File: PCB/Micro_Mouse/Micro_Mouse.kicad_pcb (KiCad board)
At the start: 2 copper layers, 88.9 x 91.4 mm, 9 parts, among them J1 Motor Battery Pack, J3 MOT_1/ENC_1, J4 MOT2/ENC_2, J5 TOF, J6 IR_1, J7 IR_2, J8 IMU, U1 TB6612FNG

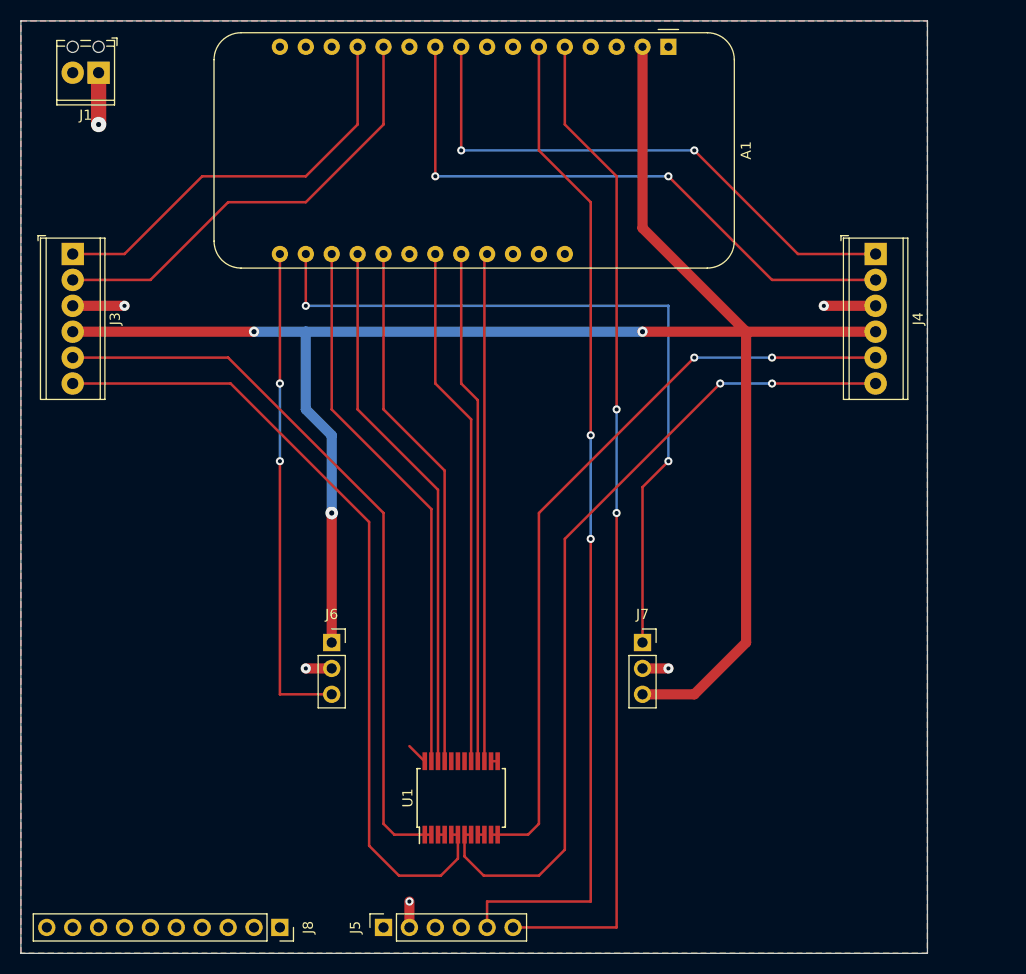
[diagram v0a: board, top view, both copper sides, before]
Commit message: Add files via upload
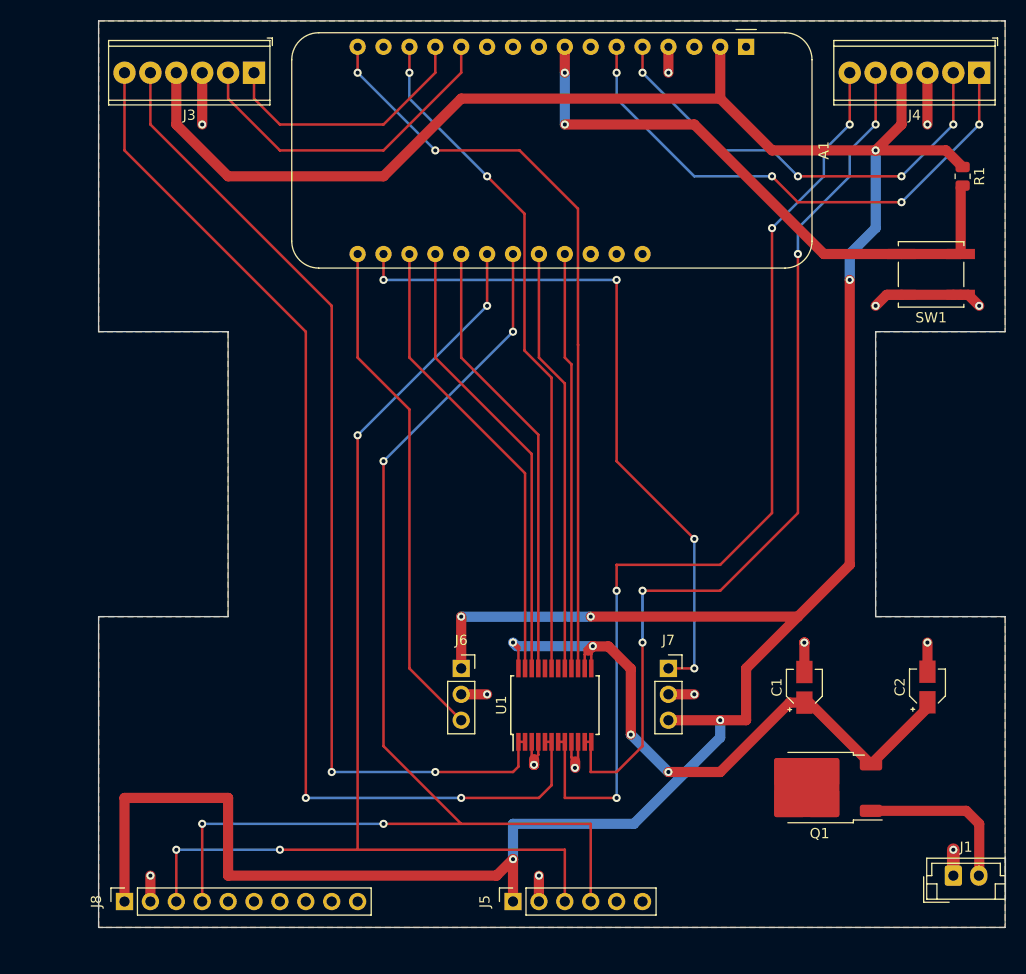
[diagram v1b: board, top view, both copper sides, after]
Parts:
- added C1: 0.1uF, Capacitor_SMD:CP_Elec_3x5.3, F.Cu at (178.4, 116.2)
- added C2: 10uF, Capacitor_SMD:CP_Elec_3x5.3, F.Cu at (190.5, 116.1)
- added Q1: PMOS, Package_TO_SOT_SMD:TO-252-2, F.Cu at (179.9, 126.0)
- added R1: 10K, Resistor_SMD:R_0805_2012Metric, F.Cu at (194.0, 66.0)
- added SW1: Start, Button_Switch_SMD:SW_Push_1P1T_NO_CK_KSC6xxJ, F.Cu at (190.9, 75.7)
- J1: footprint TerminalBlock_Phoenix:TerminalBlock_Phoenix_MPT-0,5-2-2.54_1x02_P2.54mm_Horizontal -> Connector_JST:JST_EH_B2B-EH-A_1x02_P2.50mm_Vertical
- moved J1 115.0 mm to (193.0, 134.6), turned to 0 degrees
- moved J3 25.1 mm to (124.5, 55.9), turned to 180 degrees
- moved J4 20.5 mm to (195.6, 55.9), turned to 180 degrees
- moved J8 15.5 mm to (111.8, 137.2), turned to 90 degrees
- moved J5 13.0 mm to (149.9, 137.2)
- moved J6 13.0 mm to (144.8, 114.3)
- moved U1 12.9 mm to (154.0, 117.9)
- moved A1 7.62 mm to (172.7, 53.3)
- moved J7 3.59 mm to (165.1, 114.3)
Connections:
- net Net-(A1-SCL/IO22) renamed IR_2
- net Net-(A1-SDA/IO23) renamed IR_1
- A1 pad 10: E2_PHA -> unconnected-(A1-IO4/A5-Pad10)
- A1 pad 14: unconnected-(A1-RX/IO16-Pad14) -> STBY
- A1 pad 16: unconnected-(A1-IO21-Pad16) -> PWMB
- A1 pad 22: unconnected-(A1-A9/IO33-Pad22) -> I2C SCL
- A1 pad 23: BIN1 -> I2C SDA
- A1 pad 24: BIN2 -> BIN1
- A1 pad 25: PWMB -> BIN2
- A1 pad 5: Net-(A1-DAC2/A0) -> E2_PHA
- A1 pad 6: Net-(A1-DAC1/A1) -> E2_PHB
- A1 pad 8: unconnected-(A1-I39/A3-Pad8) -> BTN
- A1 pad 9: E2_PHB -> unconnected-(A1-IO36/A4-Pad9)
- J5 pad 3: unconnected-(J5-Pin_3-Pad3) -> I2C SCL
- J5 pad 4: unconnected-(J5-Pin_4-Pad4) -> I2C SDA
- J5 pad 5: Net-(A1-DAC1/A1) -> unconnected-(J5-Pin_5-Pad5)
- J5 pad 6: Net-(A1-DAC2/A0) -> unconnected-(J5-Pin_6-Pad6)
- J8 pad 1: unconnected-(J8-Pin_1-Pad1) -> +3.3V
- J8 pad 2: unconnected-(J8-Pin_2-Pad2) -> GND
- J8 pad 3: unconnected-(J8-Pin_3-Pad3) -> I2C SCL
- J8 pad 4: unconnected-(J8-Pin_4-Pad4) -> I2C SDA
- U1 pad 13: Net-(J1-Pin_2) -> Net-(Q1-S)
- U1 pad 14: Net-(J1-Pin_2) -> Net-(Q1-S)
- U1 pad 19: unconnected-(U1-STBY-Pad19) -> STBY
- U1 pad 24: Net-(J1-Pin_2) -> Net-(Q1-S)
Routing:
- net I2C SDA: track 0.00 -> 117.6 mm, vias 0 -> 4
- net +3.3V: track 185.2 -> 300.6 mm, vias 3 -> 6
- net I2C SCL: track 0.00 -> 111.9 mm, vias 0 -> 4
- net Net-(A1-DAC2/A0): track 98.6 -> 0.00 mm, vias 2 -> 0
- net Net-(A1-DAC1/A1): track 98.6 -> 0.00 mm, vias 2 -> 0
- net STBY: track 0.00 -> 66.7 mm, vias 0 -> 2
- net Net-(Q1-S): track 0.00 -> 65.0 mm, vias 0 -> 4
- net BTN: track 0.00 -> 58.5 mm, vias 0 -> 2
- net AO2: track 80.1 -> 108.0 mm, vias 0 -> 2
- net GND: track 24.2 -> 51.3 mm, vias 6 -> 14
- net AO1: track 72.4 -> 97.6 mm, vias 0 -> 2
- net PWMB: track 49.8 -> 74.8 mm, vias 0 -> 2
- net BO2: track 81.7 -> 97.8 mm, vias 2 -> 4
- net E2_PHA: track 60.1 -> 44.4 mm, vias 2 -> 4
- net E1_PHB: track 40.8 -> 26.0 mm
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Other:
- board size 88.9 x 91.4 mm -> 88.9 x 88.9 mm
